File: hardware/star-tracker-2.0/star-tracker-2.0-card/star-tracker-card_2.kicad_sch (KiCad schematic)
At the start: 88 parts, among them Q1 DMP2240UDM, Q2 DMN3028LQ-7, Q3 DMP3050LVT-7, Q4 DMP3050LVT-7, Q5 DMN3028LQ-7, U1 MAX7310ATE, U2 MIC842LYC5, U3 MIC842LYC5, U4 TPS62112, U5 TS5A21366DCUR, U6 MAX4211FETE

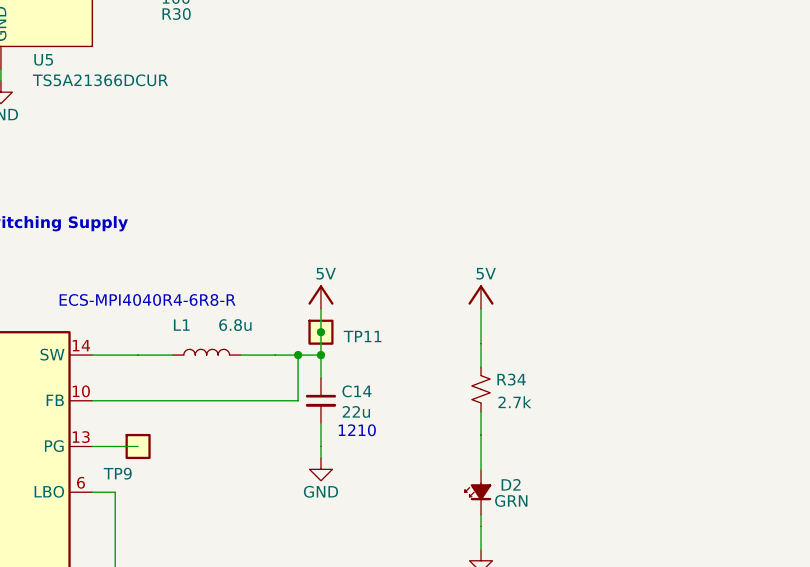
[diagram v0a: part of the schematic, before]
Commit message: Added extra Testpoints
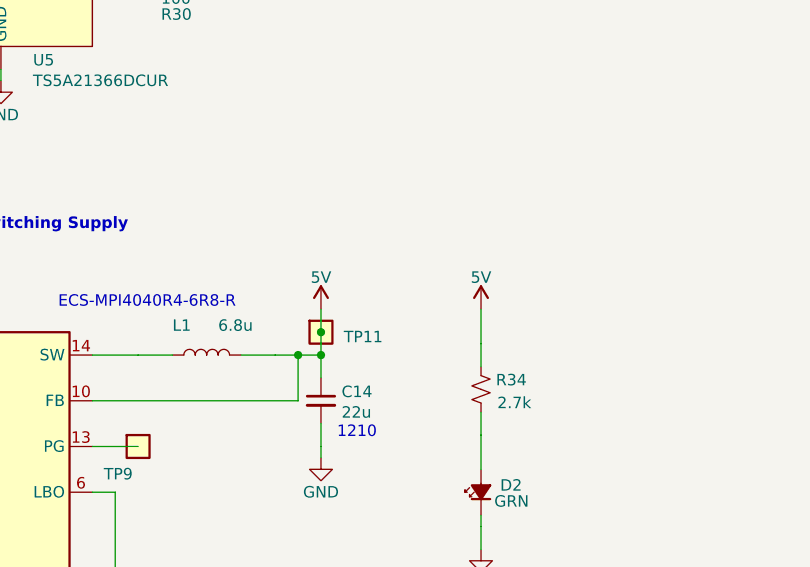
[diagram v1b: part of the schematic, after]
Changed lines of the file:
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@@
 	)
 	(symbol
-		(lib_id "star-tracker-card-eagle-import:5V")
-		(at 276.86 194.31 0)
-		(unit 1)
-		(body_style 1)
-		(exclude_from_sim no)
-		(in_bom yes)
-		(on_board yes)
-		(in_pos_files yes)
-		(dnp no)
-		(property "Reference" "#3V-02"
-			(at 276.86 194.31 0)
-			(hide yes)
-			(show_name no)
-			(do_not_autoplace no)
-			(effects
-				(font
-					(size 1.27 1.27)
-				)
-			)
-		)
-		(property "Value" "5V"
-			(at 276.225 193.675 0)
-			(show_name no)
-			(do_not_autoplace no)
-			(effects
-				(font
-					(size 1.27 1.27)
-				)
-				(justify left bottom)
-			)
-		)
-		(property "Footprint" ""
-			(at 276.86 194.31 0)
-			(hide yes)
-			(show_name no)
-			(do_not_autoplace no)
-			(effects
-				(font
-					(size 1.27 1.27)
-				)
-			)
-		)
-		(property "Datasheet" ""
-			(at 276.86 194.31 0)
-			(hide yes)
-			(show_name no)
-			(do_not_autoplace no)
-			(effects
-				(font
-					(size 1.27 1.27)
-				)
-			)
-		)
-		(property "Description" ""
-			(at 276.86 194.31 0)
-			(hide yes)
-			(show_name no)
-			(do_not_autoplace no)
-			(effects
-				(font
-					(size 1.27 1.27)
-				)
-			)
-		)
-		(pin "1"
-		)
-		(instances
-			(project "star-tracker-card"
-				(path "/324e9eb5-7420-4b7e-862c-cc20bb28618a/79e6f5da-9b7e-4636-a735-d76e4a141190"
-					(reference "#3V-02")
-					(unit 1)
-				)
-			)
-		)
-	)
-	(symbol
 		(lib_id "star-tracker-card-eagle-import:VPD")
 		(at 381 72.39 0)
@@
 	)
 	(symbol
+		(lib_id "star-tracker-card-eagle-import:VDD")
+		(at 294.64 196.85 0)
+		(unit 1)
+		(body_style 1)
+		(exclude_from_sim no)
+		(in_bom yes)
+		(on_board yes)
+		(in_pos_files yes)
+		(dnp no)
+		(property "Reference" "#SUPPLY04"
+			(at 294.64 196.85 0)
+			(hide yes)
+			(show_name no)
+			(do_not_autoplace no)
+			(effects
+				(font
+					(size 1.27 1.27)
+				)
+			)
+		)
+		(property "Value" "5V"
+			(at 294.64 194.056 0)
+			(show_name no)
+			(do_not_autoplace no)
+			(effects
+				(font
+					(size 1.27 1.27)
+				)
+				(justify bottom)
+			)
+		)
+		(property "Footprint" ""
+			(at 294.64 196.85 0)
+			(hide yes)
+			(show_name no)
+			(do_not_autoplace no)
+			(effects
+				(font
+					(size 1.27 1.27)
+				)
+			)
+		)
+		(property "Datasheet" ""
+			(at 294.64 196.85 0)
+			(hide yes)
+			(show_name no)
+			(do_not_autoplace no)
+			(effects
+				(font
+					(size 1.27 1.27)
+				)
+			)
+		)
+		(property "Description" ""
+			(at 294.64 196.85 0)
+			(hide yes)
+			(show_name no)
+			(do_not_autoplace no)
+			(effects
+				(font
+					(size 1.27 1.27)
+				)
+			)
+		)
+		(pin "1"
+		)
+		(instances
+			(project "star-tracker-card"
+				(path "/324e9eb5-7420-4b7e-862c-cc20bb28618a/79e6f5da-9b7e-4636-a735-d76e4a141190"
+					(reference "#SUPPLY04")
+					(unit 1)
+				)
+			)
+		)
+	)
+	(symbol
 		(lib_id "power:GND")
 		(at 238.76 232.41 0)
@@
 	)
 	(symbol
+		(lib_id "star-tracker-card-eagle-import:VDD")
+		(at 276.86 196.85 0)
+		(unit 1)
+		(body_style 1)
+		(exclude_from_sim no)
+		(in_bom yes)
+		(on_board yes)
+		(in_pos_files yes)
+		(dnp no)
+		(property "Reference" "#SUPPLY03"
+			(at 276.86 196.85 0)
+			(hide yes)
+			(show_name no)
+			(do_not_autoplace no)
+			(effects
+				(font
+					(size 1.27 1.27)
+				)
+			)
+		)
+		(property "Value" "5V"
+			(at 276.86 194.056 0)
+			(show_name no)
+			(do_not_autoplace no)
+			(effects
+				(font
+					(size 1.27 1.27)
+				)
+				(justify bottom)
+			)
+		)
+		(property "Footprint" ""
+			(at 276.86 196.85 0)
+			(hide yes)
+			(show_name no)
+			(do_not_autoplace no)
+			(effects
+				(font
+					(size 1.27 1.27)
+				)
+			)
+		)
+		(property "Datasheet" ""
+			(at 276.86 196.85 0)
+			(hide yes)
+			(show_name no)
+			(do_not_autoplace no)
+			(effects
+				(font
+					(size 1.27 1.27)
+				)
+			)
+		)
+		(property "Description" ""
+			(at 276.86 196.85 0)
+			(hide yes)
+			(show_name no)
+			(do_not_autoplace no)
+			(effects
+				(font
+					(size 1.27 1.27)
+				)
+			)
+		)
+		(pin "1"
+		)
+		(instances
+			(project "star-tracker-card"
+				(path "/324e9eb5-7420-4b7e-862c-cc20bb28618a/79e6f5da-9b7e-4636-a735-d76e4a141190"
+					(reference "#SUPPLY03")
+					(unit 1)
+				)
+			)
+		)
+	)
+	(symbol
 		(lib_id "star-tracker-card-eagle-import:TEST-POINT")
 		(at 100.33 130.81 0)
@@
 					(unit 1)
 				)
-			)
-		)
-	)
-	(symbol
-		(lib_id "star-tracker-card-eagle-import:5V")
-		(at 294.64 194.31 0)
-		(unit 1)
-		(body_style 1)
-		(exclude_from_sim no)
-		(in_bom yes)
-		(on_board yes)
-		(in_pos_files yes)
-		(dnp no)
-		(property "Reference" "#3V-03"
-			(at 294.64 194.31 0)
-			(hide yes)
-			(show_name no)
-			(do_not_autoplace no)
-			(effects
-				(font
-					(size 1.27 1.27)
-				)
-			)
-		)
-		(property "Value" "5V"
-			(at 294.005 193.675 0)
-			(show_name no)
-			(do_not_autoplace no)
-			(effects
-				(font
-					(size 1.27 1.27)
-				)
-				(justify left bottom)
-			)
-		)
-		(property "Footprint" ""
-			(at 294.64 194.31 0)
-			(hide yes)
-			(show_name no)
-			(do_not_autoplace no)
-			(effects
-				(font
-					(size 1.27 1.27)
-				)
-			)
-		)
-		(property "Datasheet" ""
-			(at 294.64 194.31 0)
-			(hide yes)
-			(show_name no)
-			(do_not_autoplace no)
-			(effects
-				(font
-					(size 1.27 1.27)
-				)
-			)
-		)
-		(property "Description" ""
-			(at 294.64 194.31 0)
-			(hide yes)
-			(show_name no)
-			(do_not_autoplace no)
-			(effects
-				(font
-					(size 1.27 1.27)
-				)
-			)
-		)
-		(pin "1"
-		)
-		(instances
-			(project "star-tracker-card"
-				(path "/324e9eb5-7420-4b7e-862c-cc20bb28618a/79e6f5da-9b7e-4636-a735-d76e4a141190"
-					(reference "#3V-03")
-					(unit 1)
-				)
